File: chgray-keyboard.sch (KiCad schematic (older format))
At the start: 1 part

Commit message: renaming project
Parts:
- removed U?: Teensy3.5, symbol Teensy3.5
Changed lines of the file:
@@
 Comment4 ""
 $EndDescr
-$Comp
-L Teensy3.5 U?
-U 1 1 589637DB
-P 2000 3750
-F 0 "U?" H 2000 6050 60  0000 C CNN
-F 1 "Teensy3.5" H 2000 1450 60  0000 C CNN
-F 2 "" H 2000 3750 60  0000 C CNN
-F 3 "" H 2000 3750 60  0000 C CNN
-	1    2000 3750
-	1    0    0    -1
-$EndComp
 $EndSCHEMATC

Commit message: Created Part for NXP PCA9532 BS
http://www.nxp.com/products/interfaces/ic-bus-portfolio/ic-led-display-control/16-bit-i2c-bus-led-dimmer:PCA9532BS?tab=Documentation_Tab
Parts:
- added U?: Teensy3.5, symbol Teensy3.5
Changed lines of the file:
@@
 LIBS:switches
 LIBS:teensy
+LIBS:components
+LIBS:NXP-chgray
+LIBS:chgray-keyboard-cache
 EELAYER 25 0
 EELAYER END
-$Descr A4 11693 8268
+$Descr A 11000 8500
 encoding utf-8
 Sheet 1 1
@@
 Comment4 ""
 $EndDescr
+$Comp
+L Teensy3.5 U?
+U 1 1 589644C0
+P 1700 3550
+F 0 "U?" H 1700 5850 60  0000 C CNN
+F 1 "Teensy3.5" H 1700 1250 60  0000 C CNN
+F 2 "" H 1700 3550 60  0000 C CNN
+F 3 "" H 1700 3550 60  0000 C CNN
+	1    1700 3550
+	1    0    0    -1
+$EndComp
 $EndSCHEMATC

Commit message: placing parts
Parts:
- U1: renamed from U?; footprint (none) -> Teensy:Teensy35_36
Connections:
- wire segments 0 -> 45
- no-connect marks 0 -> 73
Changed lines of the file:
@@
 $Descr A 11000 8500
 encoding utf-8
-Sheet 1 1
+Sheet 1 3
 Title ""
 Date ""
@@
 Comment4 ""
 $EndDescr
+$Sheet
+S 7300 1800 2100 1850
+U 589645BF
+F0 "Keyboard Keys" 60
+F1 "Keys.sch" 60
+F2 "KEY_COL0" I L 7300 2000 60
+F3 "KEY_ROW0" I R 9400 1950 60
+F4 "KEY_ROW1" I R 9400 2150 60
+F5 "KEY_COL1" I L 7300 2150 60
+F6 "KEY_COL2" I L 7300 2300 60
+F7 "KEY_COL3" I L 7300 2450 60
+F8 "KEY_COL4" I L 7300 2600 60
+F9 "KEY_COL5" I L 7300 2750 60
+F10 "KEY_COL6" I L 7300 2900 60
+F11 "KEY_COL7" I L 7300 3050 60
+F12 "KEY_COL8" I L 7300 3200 60
+$EndSheet
+$Sheet
+S 4550 3950 2450 1950
+U 589645DC
+F0 "Keyboard LEDS" 60
+F1 "LEDs.sch" 60
+F2 "I2C_CLK" I L 4550 4250 60
+F3 "I2C_DTA" I L 4550 4450 60
+$EndSheet
+NoConn ~ 1850 3050
+NoConn ~ 1850 4050
+NoConn ~ 1850 4150
+NoConn ~ 1850 4250
+NoConn ~ 1850 4350
+NoConn ~ 1850 4450
+NoConn ~ 1850 4550
+NoConn ~ 1850 4650
+NoConn ~ 1850 4750
+NoConn ~ 1850 4850
+NoConn ~ 1850 4950
+NoConn ~ 1850 5050
+NoConn ~ 1850 5150
+NoConn ~ 1850 5450
+NoConn ~ 1850 5550
+NoConn ~ 1850 5650
+NoConn ~ 1850 5750
+NoConn ~ 1850 5850
+NoConn ~ 1850 5950
+NoConn ~ 1850 6250
+NoConn ~ 1850 6350
+NoConn ~ 1850 6450
+NoConn ~ 1850 6550
+NoConn ~ 1850 6650
+NoConn ~ 1850 6750
+NoConn ~ 1850 6850
+NoConn ~ 1850 6950
+NoConn ~ 1850 7050
+NoConn ~ 1850 7150
+NoConn ~ 1850 7250
+NoConn ~ 3850 3250
+NoConn ~ 3850 3350
+NoConn ~ 3850 3450
+NoConn ~ 3850 3550
+NoConn ~ 3850 3650
+NoConn ~ 3850 3750
+NoConn ~ 3850 3850
+NoConn ~ 3850 3950
+NoConn ~ 3850 4050
+NoConn ~ 3850 4150
+NoConn ~ 3850 4250
+NoConn ~ 3850 4350
+NoConn ~ 3850 4450
+NoConn ~ 3850 4550
+NoConn ~ 3850 4650
+NoConn ~ 3850 4750
+NoConn ~ 3850 4850
+NoConn ~ 3850 4950
+NoConn ~ 3850 5050
+NoConn ~ 3850 5150
+NoConn ~ 3850 5250
+NoConn ~ 3850 5350
+NoConn ~ 3850 5450
+NoConn ~ 3850 5550
+NoConn ~ 3850 5650
+NoConn ~ 3850 5750
+NoConn ~ 3850 5850
+NoConn ~ 3850 5950
+NoConn ~ 3850 6050
+NoConn ~ 3850 6150
+NoConn ~ 3850 6250
+NoConn ~ 3850 6350
+NoConn ~ 3850 6450
+NoConn ~ 3850 6550
+NoConn ~ 3850 6650
+NoConn ~ 3850 6750
+NoConn ~ 3850 6850
+NoConn ~ 3850 6950
+NoConn ~ 3850 7050
+NoConn ~ 3850 7150
+NoConn ~ 3850 7250
+NoConn ~ 3850 3050
+NoConn ~ 3850 3150
+Wire Wire Line
+	7300 2000 1650 850
+Wire Wire Line
+	1650 850  1650 1950
+Wire Wire Line
+	1650 1950 1850 3150
+Wire Wire Line
+	1850 3250 1600 2050
+Wire Wire Line
+	1600 2050 1600 1000
+Wire Wire Line
+	1600 1000 7300 2150
+Wire Wire Line
+	7300 2300 1450 1150
+Wire Wire Line
+	1450 1150 1450 2150
+Wire Wire Line
+	1450 2150 1850 3350
+Wire Wire Line
+	7300 2450 1350 1300
+Wire Wire Line
+	1350 1300 1350 2250
+Wire Wire Line
+	1350 2250 1850 3450
+Wire Wire Line
+	7300 2600 1100 1450
+Wire Wire Line
+	1100 1450 1100 2350
+Wire Wire Line
+	1100 2350 1850 3550
+Wire Wire Line
+	7300 2750 900  1600
+Wire Wire Line
+	900  1600 900  2450
+Wire Wire Line
+	900  2450 1850 3650
+Wire Wire Line
+	7300 2900 850  1750
+Wire Wire Line
+	850  1750 850  2550
+Wire Wire Line
+	850  2550 1850 3750
+Wire Wire Line
+	7300 3050 750  1900
+Wire Wire Line
+	750  1900 750  2650
+Wire Wire Line
+	750  2650 1850 3850
+Wire Wire Line
+	7300 3200 550  2050
+Wire Wire Line
+	550  2050 550  2750
+Wire Wire Line
+	550  2750 1850 3950
+Wire Wire Line
+	9400 1950 750  800
+Wire Wire Line
+	750  800  750  5250
+Wire Wire Line
+	750  5250 1850 5250
+Wire Wire Line
+	1850 5350 650  5350
+Wire Wire Line
+	650  5350 650  1100
+Wire Wire Line
+	650  1100 7250 1100
+Wire Wire Line
+	7250 1100 7250 1000
+Wire Wire Line
+	7250 1000 9400 2150
 $Comp
-L Teensy3.5 U?
+L Teensy3.5 U1
 U 1 1 589644C0
-P 1700 3550
-F 0 "U?" H 1700 5850 60  0000 C CNN
-F 1 "Teensy3.5" H 1700 1250 60  0000 C CNN
-F 2 "" H 1700 3550 60  0000 C CNN
-F 3 "" H 1700 3550 60  0000 C CNN
-	1    1700 3550
+P 2850 5150
+F 0 "U1" H 2850 7450 60  0000 C CNN
+F 1 "Teensy3.5" H 2850 2850 60  0000 C CNN
+F 2 "Teensy:Teensy35_36" H 2850 5150 60  0001 C CNN
+F 3 "" H 2850 5150 60  0000 C CNN
+	1    2850 5150
 	1    0    0    -1
 $EndComp
+Wire Wire Line
+	1850 6050 1550 6050
+Wire Wire Line
+	1550 6050 1550 7700
+Wire Wire Line
+	1550 7700 4300 7700
+Wire Wire Line
+	4300 7700 4300 4250
+Wire Wire Line
+	4300 4250 4550 4250
+Wire Wire Line
+	4550 4450 4150 4450
+Wire Wire Line
+	4150 4450 4150 7800
+Wire Wire Line
+	4150 7800 1400 7800
+Wire Wire Line
+	1400 7800 1400 6150
+Wire Wire Line
+	1400 6150 1850 6150
 $EndSCHEMATC

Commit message: test keyboard
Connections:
- wire segments 45 -> 16
- no-connect marks 73 -> 82

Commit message: messing around
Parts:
- U1: symbol Teensy3.5 -> chgray-keyboard-rescue:Teensy3.5-
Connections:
- wire segments 16 -> 21
- no-connect marks 82 -> 81
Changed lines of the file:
@@
-EESchema Schematic File Version 2
-LIBS:power
-LIBS:device
-LIBS:switches
-LIBS:teensy
-LIBS:components
-LIBS:NXP-chgray
-LIBS:chgray-keyboard-cache
-EELAYER 25 0
+EESchema Schematic File Version 4
+EELAYER 30 0
 EELAYER END
 $Descr A 11000 8500
@@
 F4 "KEY_ROW1" I R 9400 2150 60
 F5 "KEY_COL1" I L 7300 2150 60
+F6 "KEY_ROW2" I R 9400 2350 50
 $EndSheet
 NoConn ~ 2250 2750
@@
 NoConn ~ 2250 4650
 NoConn ~ 2250 4750
-NoConn ~ 2250 4850
 NoConn ~ 2250 5150
 NoConn ~ 2250 5250
@@
 NoConn ~ 4250 2850
 $Comp
-L Teensy3.5 U1
+L chgray-keyboard-rescue:Teensy3.5- U1
 U 1 1 589644C0
 P 3250 4850
@@
 Wire Wire Line
 	1500 3850 1500 2150
-Connection ~ 1500 2150
 Wire Wire Line
 	1500 2150 7300 2150
 NoConn ~ 2250 4050
 NoConn ~ 2250 4150
+Wire Wire Line
+	9400 2350 9950 2350
+Wire Wire Line
+	9950 2350 9950 1000
+Wire Wire Line
+	9950 1000 1000 1000
+Wire Wire Line
+	1000 1000 1000 4850
+Wire Wire Line
+	1000 4850 2250 4850
 $EndSCHEMATC

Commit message: working
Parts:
- U1: footprint Teensy:Teensy35_36 -> Teensy_Pretty:Teensy35_36
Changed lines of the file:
@@
 F 0 "U1" H 3250 7150 60  0000 C CNN
 F 1 "Teensy3.5" H 3250 2550 60  0000 C CNN
-F 2 "Teensy:Teensy35_36" H 3250 4850 60  0001 C CNN
+F 2 "Teensy_Pretty:Teensy35_36" H 3250 4850 60  0001 C CNN
 F 3 "" H 3250 4850 60  0000 C CNN
 	1    3250 4850

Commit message: docker file
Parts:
- U1: symbol chgray-keyboard-rescue:Teensy3.5- -> chgray-keyboard-rescue:Teensy3.5--chgray-keyboard-rescue
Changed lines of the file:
@@
 NoConn ~ 4250 2850
 $Comp
-L chgray-keyboard-rescue:Teensy3.5- U1
+L chgray-keyboard-rescue:Teensy3.5--chgray-keyboard-rescue U1
 U 1 1 589644C0
 P 3250 4850

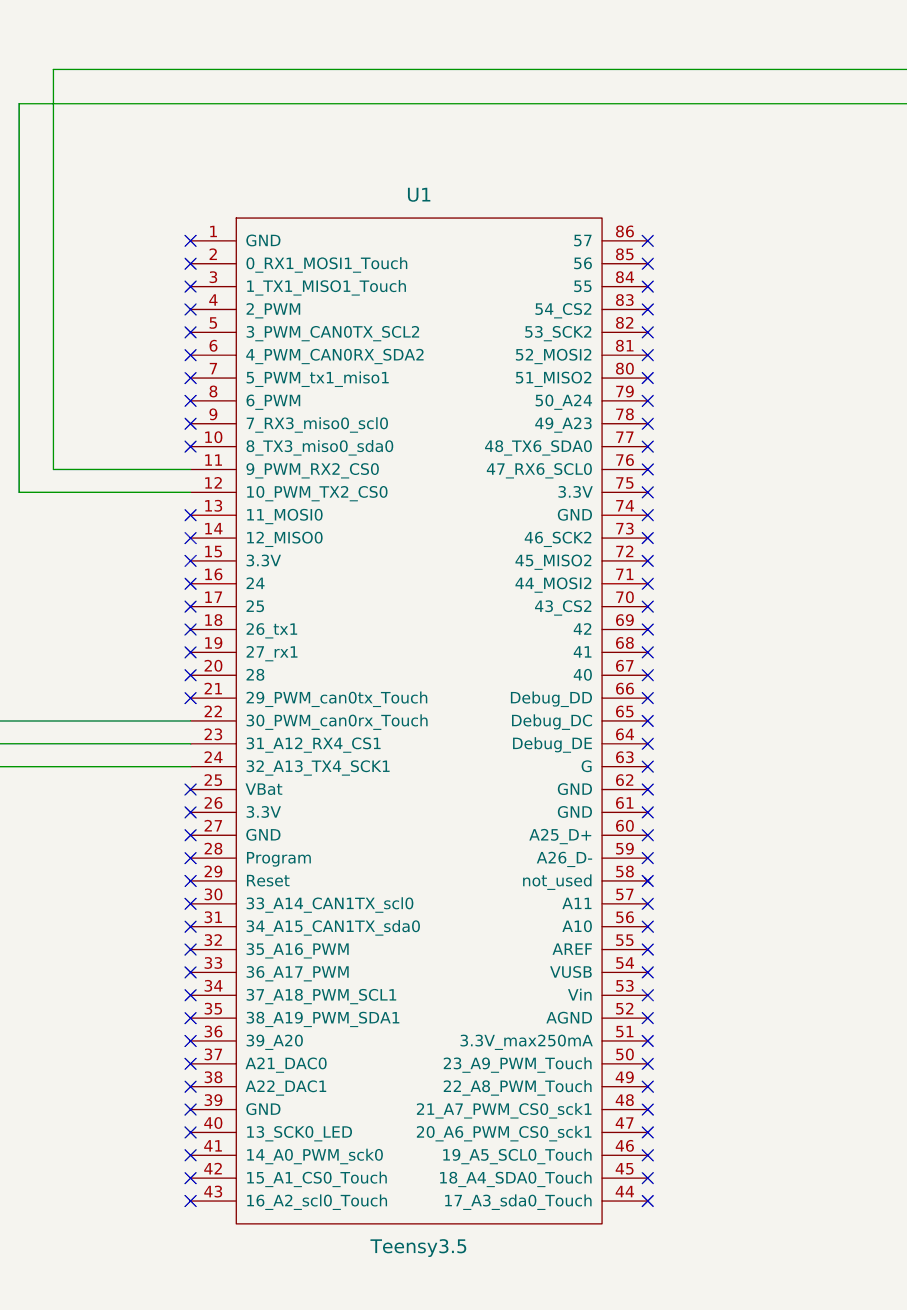
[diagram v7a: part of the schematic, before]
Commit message: working
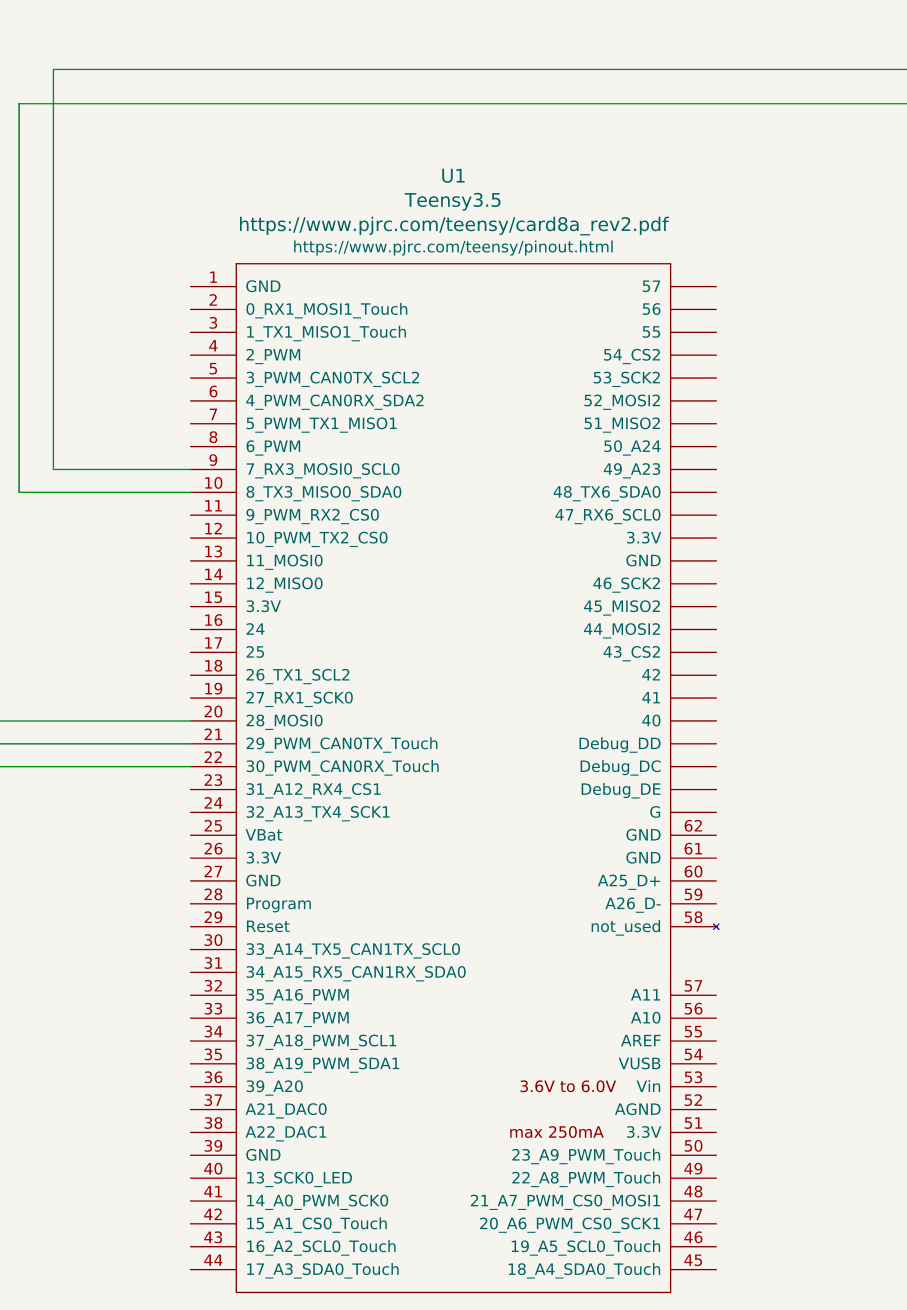
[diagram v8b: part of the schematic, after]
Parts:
- removed U1: Teensy3.5, Teensy_Pretty:Teensy35_36, symbol chgray-keyboard-rescue:Teensy3.5--chgray-keyboard-rescue
- added U1: Teensy3.5, Teensy_Pretty:Teensy35_36, symbol Teensy:Teensy3.5
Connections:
- net Keyboard Keys/KEY_COL0: now also U1.9 (7_RX3_MOSI0_SCL0)
- net Keyboard Keys/KEY_COL1: now also U1.10 (8_TX3_MISO0_SDA0)
- net Keyboard Keys/KEY_ROW0: now also U1.21 (29_PWM_CAN0TX_Touch)
- net Keyboard Keys/KEY_ROW1: now also U1.22 (30_PWM_CAN0RX_Touch)
- net Keyboard Keys/KEY_ROW2: now also U1.20 (28_MOSI0)
- no-connect marks 81 -> 0
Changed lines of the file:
@@
 F6 "KEY_ROW2" I R 9400 2350 50
 $EndSheet
-NoConn ~ 2250 2750
-NoConn ~ 2250 3950
-NoConn ~ 2250 4250
-NoConn ~ 2250 4350
-NoConn ~ 2250 4450
-NoConn ~ 2250 4550
-NoConn ~ 2250 4650
-NoConn ~ 2250 4750
-NoConn ~ 2250 5150
-NoConn ~ 2250 5250
-NoConn ~ 2250 5350
-NoConn ~ 2250 5450
-NoConn ~ 2250 5550
-NoConn ~ 2250 5650
-NoConn ~ 2250 5950
-NoConn ~ 2250 6050
-NoConn ~ 2250 6150
-NoConn ~ 2250 6250
-NoConn ~ 2250 6350
-NoConn ~ 2250 6450
-NoConn ~ 2250 6550
-NoConn ~ 2250 6650
-NoConn ~ 2250 6750
-NoConn ~ 2250 6850
-NoConn ~ 2250 6950
-NoConn ~ 4250 2950
-NoConn ~ 4250 3050
-NoConn ~ 4250 3150
-NoConn ~ 4250 3250
-NoConn ~ 4250 3350
-NoConn ~ 4250 3450
-NoConn ~ 4250 3550
-NoConn ~ 4250 3650
-NoConn ~ 4250 3750
-NoConn ~ 4250 3850
-NoConn ~ 4250 3950
-NoConn ~ 4250 4050
-NoConn ~ 4250 4150
-NoConn ~ 4250 4250
-NoConn ~ 4250 4350
-NoConn ~ 4250 4450
-NoConn ~ 4250 4550
-NoConn ~ 4250 4650
-NoConn ~ 4250 4750
-NoConn ~ 4250 4850
-NoConn ~ 4250 4950
-NoConn ~ 4250 5050
-NoConn ~ 4250 5150
-NoConn ~ 4250 5250
-NoConn ~ 4250 5350
-NoConn ~ 4250 5450
-NoConn ~ 4250 5550
-NoConn ~ 4250 5650
-NoConn ~ 4250 5750
-NoConn ~ 4250 5850
-NoConn ~ 4250 5950
-NoConn ~ 4250 6050
-NoConn ~ 4250 6150
-NoConn ~ 4250 6250
-NoConn ~ 4250 6350
-NoConn ~ 4250 6450
-NoConn ~ 4250 6550
-NoConn ~ 4250 6650
-NoConn ~ 4250 6750
-NoConn ~ 4250 6850
-NoConn ~ 4250 6950
-NoConn ~ 4250 2750
-NoConn ~ 4250 2850
-$Comp
-L chgray-keyboard-rescue:Teensy3.5--chgray-keyboard-rescue U1
-U 1 1 589644C0
-P 3250 4850
-F 0 "U1" H 3250 7150 60  0000 C CNN
-F 1 "Teensy3.5" H 3250 2550 60  0000 C CNN
-F 2 "Teensy_Pretty:Teensy35_36" H 3250 4850 60  0001 C CNN
-F 3 "" H 3250 4850 60  0000 C CNN
-	1    3250 4850
-	1    0    0    -1
-$EndComp
 Wire Wire Line
 	9600 1950 9600 1500
@@
 Wire Wire Line
 	9750 1300 9750 2150
-NoConn ~ 2250 2850
-NoConn ~ 2250 2950
-NoConn ~ 2250 3050
-NoConn ~ 2250 3150
-NoConn ~ 2250 3250
-NoConn ~ 2250 3350
-NoConn ~ 2250 3450
-NoConn ~ 2250 3550
-NoConn ~ 2250 3650
 Wire Wire Line
 	1350 4950 2250 4950
 Wire Wire Line
 	2250 5050 1150 5050
-NoConn ~ 2250 5750
-NoConn ~ 2250 5850
 Wire Wire Line
 	7300 2000 1650 2000
@@
 Wire Wire Line
 	1500 2150 7300 2150
-NoConn ~ 2250 4050
-NoConn ~ 2250 4150
 Wire Wire Line
 	9400 2350 9950 2350
@@
 Wire Wire Line
 	1000 4850 2250 4850
+$Comp
+L Teensy:Teensy3.5 U1
+U 1 1 605697C1
+P 3400 5100
+F 0 "U1" H 3400 7733 60  0000 C CNN
+F 1 "Teensy3.5" H 3400 7627 60  0000 C CNN
+F 2 "Teensy_Pretty:Teensy35_36" H 3300 7350 60  0001 C CNN
+F 3 "https://www.pjrc.com/teensy/card8a_rev2.pdf" H 3400 7521 60  0000 C CNN
+F 4 "https://www.pjrc.com/teensy/pinout.html" H 3400 7423 50  0000 C CNN "Pinouts"
+	1    3400 5100
+	1    0    0    -1
+$EndComp
 $EndSCHEMATC
